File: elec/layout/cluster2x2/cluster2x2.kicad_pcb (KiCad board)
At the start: 2 copper layers, 31 parts

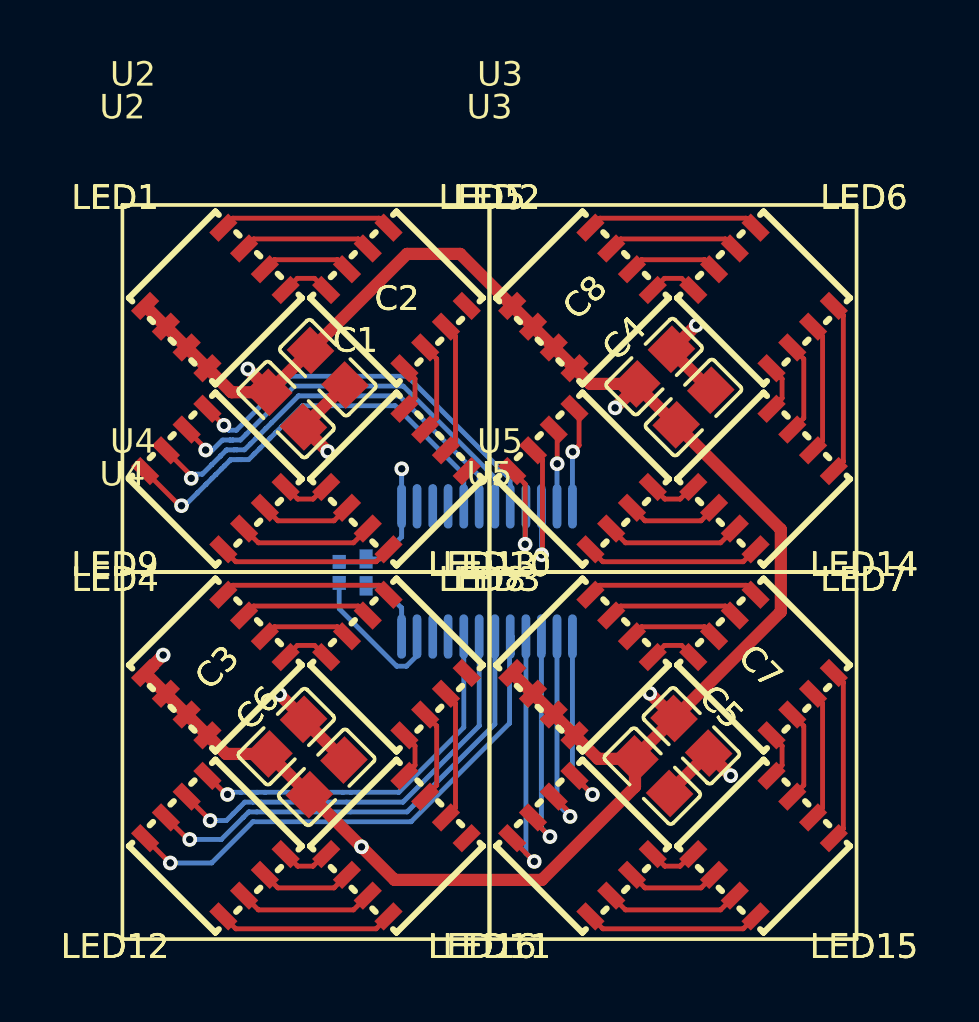
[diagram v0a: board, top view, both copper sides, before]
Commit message: shipped board
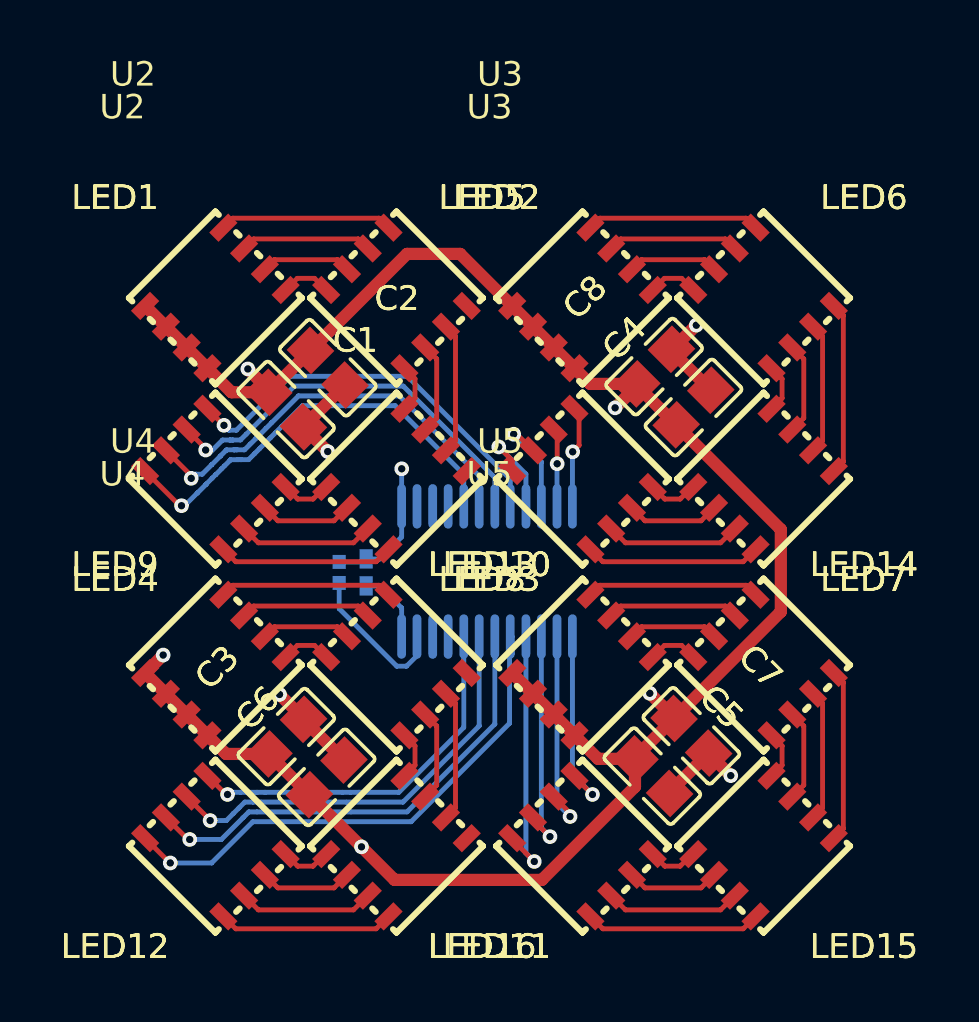
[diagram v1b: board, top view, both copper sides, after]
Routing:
- net -blue-3: track 6.43 -> 4.48 mm
- net -cold_white-3: track 4.77 -> 4.11 mm
